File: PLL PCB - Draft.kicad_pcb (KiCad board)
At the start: 4 copper layers, 82 x 44.9 mm, 78 parts, among them IC1 RRA78610-QAJ, J1 Conn_01x02_Socket, J2 Conn_01x06_Socket, J4 External_VCO_RF, J5 SMA_For_External_REF, U1 LT3045EMSE_PBF, U2 CWX813-100.0M, U3 ADP150AUJZ-1.8-R7, U8 ADP150AUJZ-3.3-R7, U9 ADP150AUJZ-3.0-R7

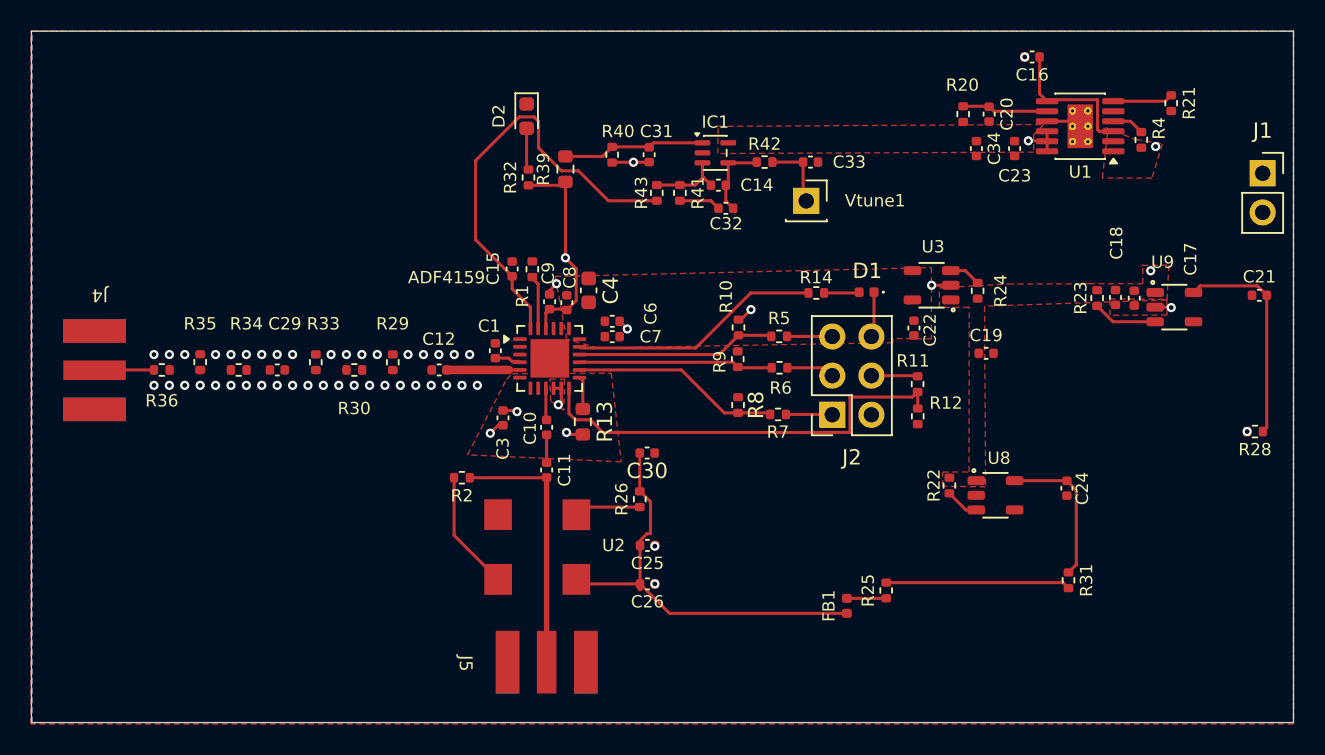
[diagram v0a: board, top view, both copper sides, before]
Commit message: complete pcb design
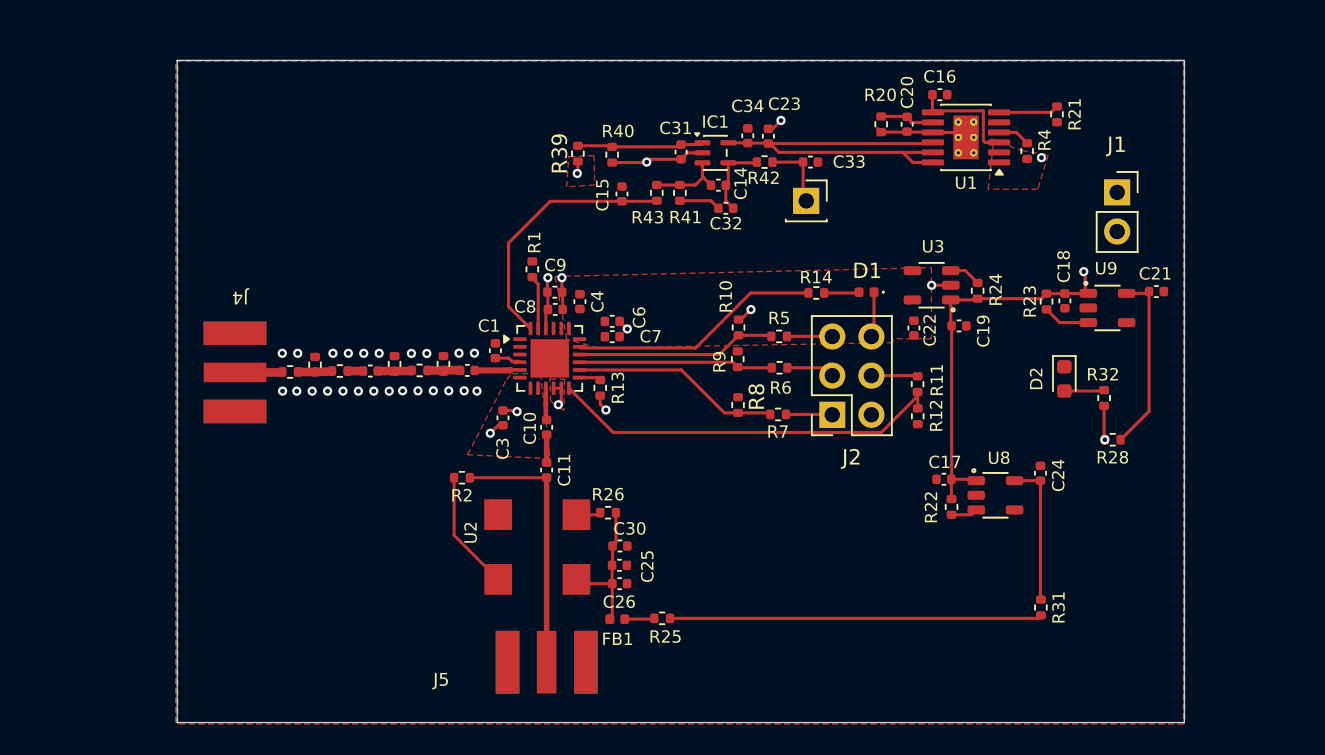
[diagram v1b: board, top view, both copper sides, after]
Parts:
- C34: value 0F -> 0.1uF
- C4: footprint Capacitor_SMD:C_0603_1608Metric -> Capacitor_SMD:C_0402_1005Metric
- R13, R39: footprint Resistor_SMD:R_0603_1608Metric -> Resistor_SMD:R_0402_1005Metric
- moved R32 40.0 mm to (204.2, 65.3)
- moved D2 38.9 mm to (201.6, 64.1)
- moved C17 17.1 mm to (193.8, 70.6), turned to 180 degrees
- moved C23 16.0 mm to (182.4, 48.3), turned to 90 degrees
- moved FB1 14.9 mm to (172.6, 79.7), turned to 0 degrees
- moved C34 14.9 mm to (181.1, 48.3), turned to 90 degrees
- moved R25 14.7 mm to (175.5, 79.6), turned to 0 degrees
- moved J1 9.53 mm to (205.1, 52.0)
- moved R28 9.26 mm to (204.8, 68.0)
- moved J4 9.12 mm to (145.7, 63.7)
- moved C15 8.63 mm to (172.9, 52.1)
- moved R36 8.33 mm to (151.3, 63.6)
- moved R35 7.46 mm to (153.0, 63.2)
- moved R21 7.45 mm to (201.1, 46.9)
- moved R4 7.45 mm to (199.2, 49.3)
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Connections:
- J4 pad GND@3: (no net) -> GND
- J4 pad GND@4: (no net) -> GND
- J5 pad GND@3: (no net) -> GND
- J5 pad GND@4: (no net) -> GND
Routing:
- net /Loop Filter/5.5V: track 2.53 -> 26.6 mm, vias 1 -> 0
- net /ADF4159/3.0V: track 27.4 -> 8.63 mm, vias 4 -> 5
- net Net-(C25-Pad2): track 27.7 -> 9.94 mm
- net /Power Supply/OSC_VDD_3.3V: track 12.0 -> 24.4 mm
- net /ADF4159/CPOUT: track 28.6 -> 16.9 mm
- net GND: track 12.9 -> 21.7 mm, vias 51 -> 32
- net /+6.5V_RAW: track 27.1 -> 33.5 mm
- net Net-(R26-Pad1): track 4.32 -> 1.60 mm
- net Net-(C12-Pad2): track 4.53 -> 2.15 mm
- net Net-(U9-VOUT): track 14.1 -> 11.9 mm
- net Net-(ADF4159-TXDATA): track 28.3 -> 26.2 mm
- net Net-(U1-SET): track 5.58 -> 3.63 mm
- net Net-(C29-Pad1): track 4.02 -> 2.24 mm
- net Net-(R34-Pad2): track 4.00 -> 2.23 mm
- net /ADF4159/RFIN: track 4.06 -> 2.35 mm
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- removed copper zone on F.Cu, net /Loop Filter/5.5V
- removed copper zone on In2.Cu, net /Loop Filter/5.5V
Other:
- board size 82 x 44.9 mm -> 65.4 x 43 mm
